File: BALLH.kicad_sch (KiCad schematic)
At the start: 5 parts

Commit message: R20260922
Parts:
- R26: footprint (none) -> Resistor_THT:R_Axial_DIN0207_L6.3mm_D2.5mm_P10.16mm_Horizontal
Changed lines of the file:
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@@
 			)
 		)
-		(property "Footprint" ""
+		(property "Footprint" "Resistor_THT:R_Axial_DIN0207_L6.3mm_D2.5mm_P10.16mm_Horizontal"
 			(at 101.346 139.954 90)
 			(hide yes)

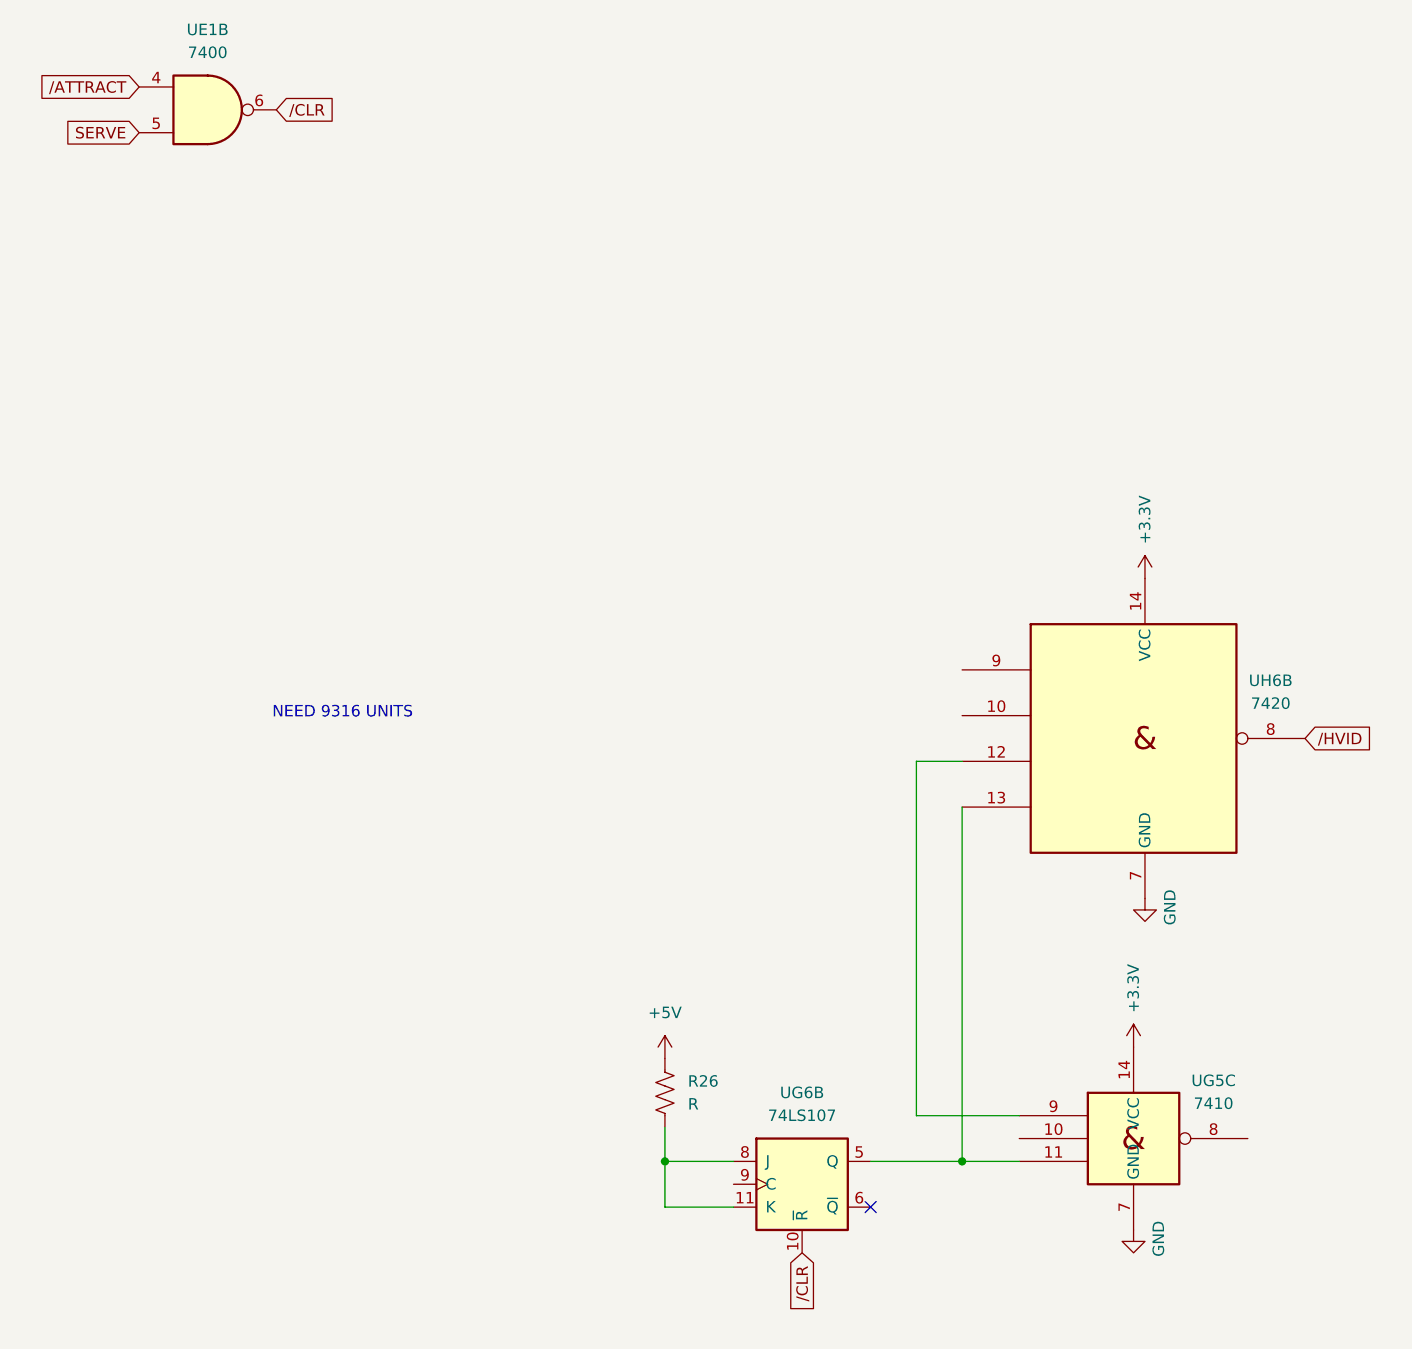
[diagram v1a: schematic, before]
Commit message: R20260922PM
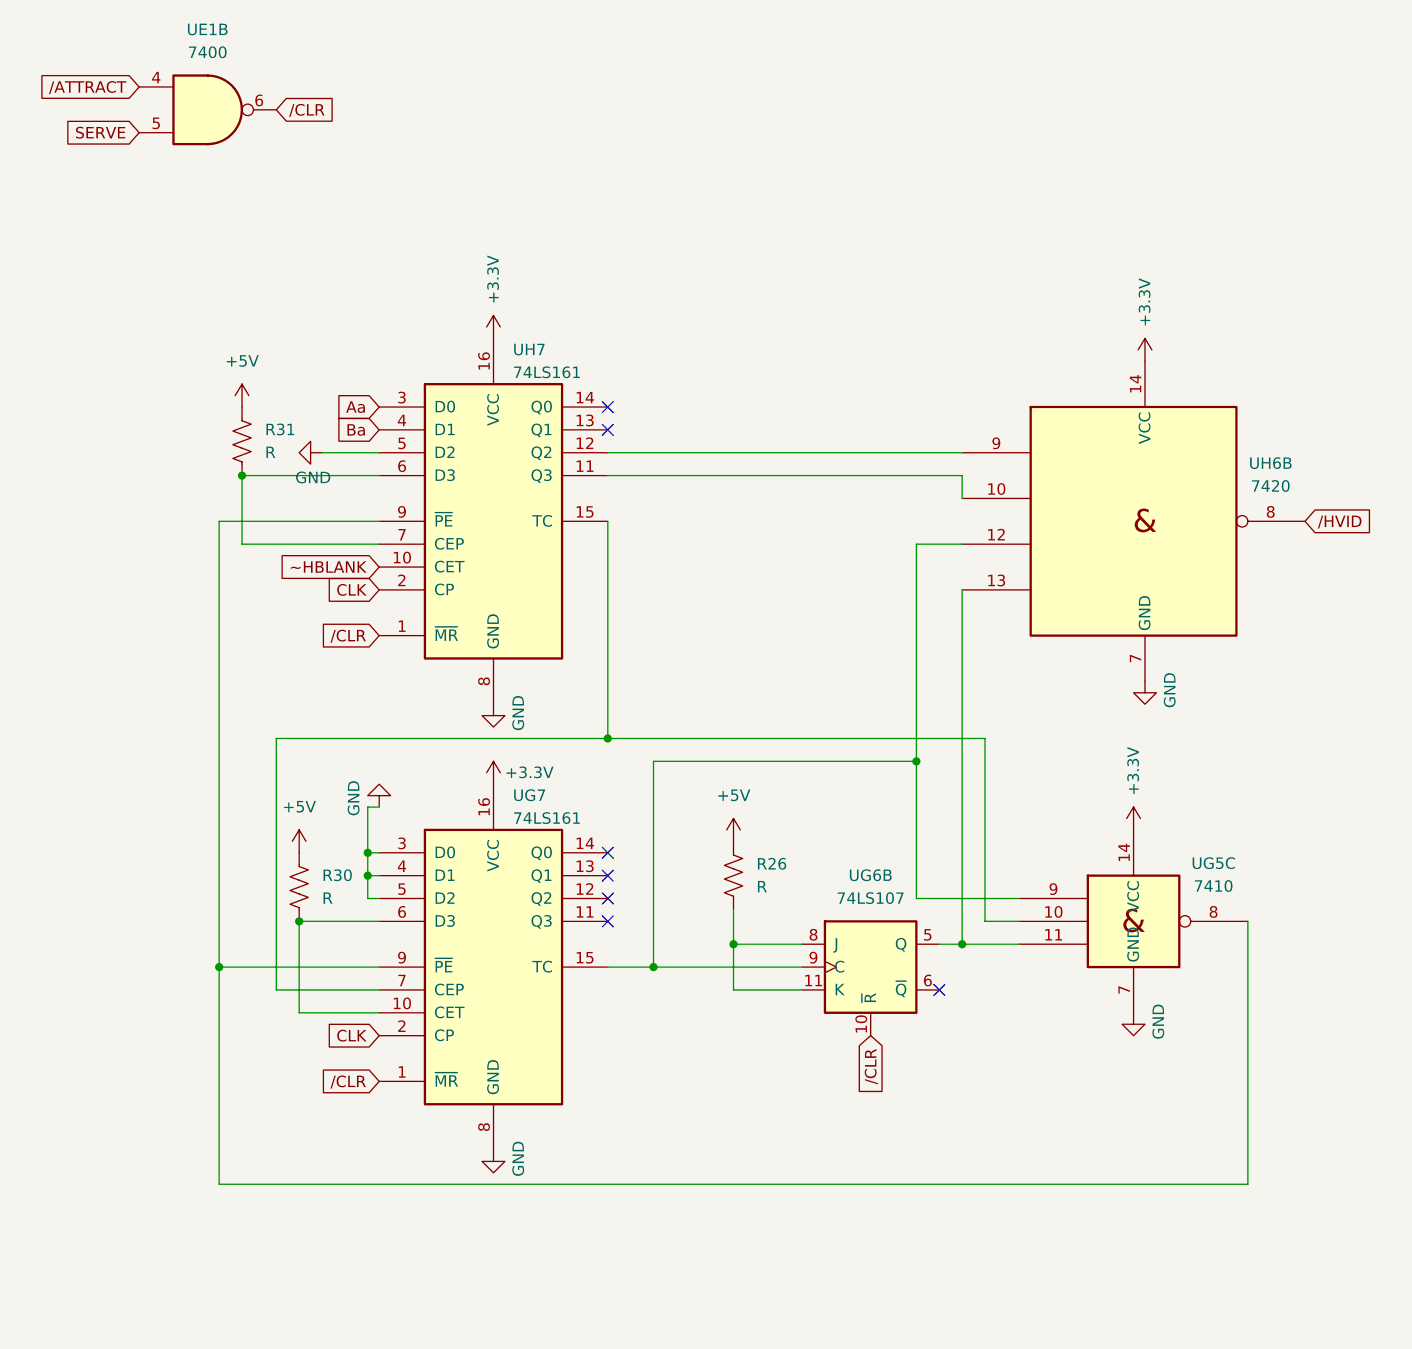
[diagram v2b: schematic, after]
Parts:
- added R30, R31: R, Resistor_THT:R_Axial_DIN0207_L6.3mm_D2.5mm_P10.16mm_Horizontal, symbol Device:R_US
- added UG7, UH7: 74LS161, pong:pong_DIP-16_W7.62mm_Socket_LongPads, symbol 74xx:74LS161
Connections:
- net +3.3V: now also UG7.16 (VCC), UH7.16 (VCC)
- net +5V: now also R30.1, R31.1
- net GND: now also UG7.3 (D0), UG7.4 (D1), UG7.5 (D2), UG7.8 (GND), UH7.5 (D2), UH7.8 (GND)
- net /CLR: now also UG7.1 (~{MR}), UH7.1 (~{MR})
- net at UG6.9 (C): now also UG5.9, UH6.12, UG7.15 (TC)
- net at UH6.10: now also UH7.11 (Q3)
- net at UH6.9: now also UH7.12 (Q2)
- net at UG5.10: now also UG7.7 (CEP), UH7.15 (TC)
- net at UG5.8: now also UG7.9 (~{PE}), UH7.9 (~{PE})
- new net: R30.2, UG7.10 (CET), UG7.6 (D3)
- new net: R31.2, UH7.6 (D3), UH7.7 (CEP)
- new net Aa: UH7.3 (D0)
- new net Ba: UH7.4 (D1)
- new net CLK: UG7.2 (CP), UH7.2 (CP)
- new net ~HBLANK: UH7.10 (CET)
- no-connect marks 1 -> 7
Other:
- note removed: "NEED 9316 UNITS"
- moved on the sheet: R26, UG5C, UG6B, UH6B
